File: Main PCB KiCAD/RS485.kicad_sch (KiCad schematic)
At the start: 5 parts, among them J8 RS485, U2 MAX3072E

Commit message: changes adn updates
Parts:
- J8: footprint Connector_Molex:Molex_Nano-Fit_105309-xx08_1x08_P2.50mm_Vertical -> Connector_JST:JST_PH_S8B-PH-K_1x08_P2.00mm_Horizontal
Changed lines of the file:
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@@
 		(dnp no)
 		(fields_autoplaced yes)
-		(property "Reference" "#PWR031"
+		(property "Reference" "#PWR03"
 			(at 217.17 123.19 0)
 			(effects
@@
 		(instances
 			(project "Buoy PCB"
-				(path "/a041e2a6-7d41-458c-91f3-753821d3dfe9/e4da0947-b13f-47c4-af36-48578442859c"
-					(reference "#PWR031")
+				(path "/a041e2a6-7d41-458c-91f3-753821d3dfe9/402c8c5f-ad4a-46d2-a42e-eba9c7fe5855/d9a8ca03-ff66-4db5-998a-66a2672c57da"
+					(reference "#PWR03")
 					(unit 1)
 				)
@@
 		)
 		(instances
-			(project ""
-				(path "/a041e2a6-7d41-458c-91f3-753821d3dfe9/e4da0947-b13f-47c4-af36-48578442859c"
+			(project "Buoy PCB"
+				(path "/a041e2a6-7d41-458c-91f3-753821d3dfe9/402c8c5f-ad4a-46d2-a42e-eba9c7fe5855/d9a8ca03-ff66-4db5-998a-66a2672c57da"
 					(reference "U2")
 					(unit 1)
@@
 		(instances
 			(project "Buoy PCB"
-				(path "/a041e2a6-7d41-458c-91f3-753821d3dfe9/e4da0947-b13f-47c4-af36-48578442859c"
+				(path "/a041e2a6-7d41-458c-91f3-753821d3dfe9/402c8c5f-ad4a-46d2-a42e-eba9c7fe5855/d9a8ca03-ff66-4db5-998a-66a2672c57da"
 					(reference "R7")
 					(unit 1)
@@
 		(instances
 			(project "Buoy PCB"
-				(path "/a041e2a6-7d41-458c-91f3-753821d3dfe9/e4da0947-b13f-47c4-af36-48578442859c"
+				(path "/a041e2a6-7d41-458c-91f3-753821d3dfe9/402c8c5f-ad4a-46d2-a42e-eba9c7fe5855/d9a8ca03-ff66-4db5-998a-66a2672c57da"
 					(reference "JP2")
 					(unit 1)
@@
 		(dnp no)
 		(fields_autoplaced yes)
-		(property "Reference" "#PWR034"
+		(property "Reference" "#PWR032"
 			(at 275.59 151.13 0)
 			(effects
@@
 		(instances
 			(project "Buoy PCB"
-				(path "/a041e2a6-7d41-458c-91f3-753821d3dfe9/e4da0947-b13f-47c4-af36-48578442859c"
-					(reference "#PWR034")
+				(path "/a041e2a6-7d41-458c-91f3-753821d3dfe9/402c8c5f-ad4a-46d2-a42e-eba9c7fe5855/d9a8ca03-ff66-4db5-998a-66a2672c57da"
+					(reference "#PWR032")
 					(unit 1)
 				)
@@
 			)
 		)
-		(property "Footprint" "Connector_Molex:Molex_Nano-Fit_105309-xx08_1x08_P2.50mm_Vertical"
+		(property "Footprint" "Connector_JST:JST_PH_S8B-PH-K_1x08_P2.00mm_Horizontal"
 			(at 283.21 132.08 0)
 			(effects
@@
 		(instances
 			(project "Buoy PCB"
-				(path "/a041e2a6-7d41-458c-91f3-753821d3dfe9/e4da0947-b13f-47c4-af36-48578442859c"
+				(path "/a041e2a6-7d41-458c-91f3-753821d3dfe9/402c8c5f-ad4a-46d2-a42e-eba9c7fe5855/d9a8ca03-ff66-4db5-998a-66a2672c57da"
 					(reference "J8")
 					(unit 1)
@@
 		(instances
 			(project "Buoy PCB"
-				(path "/a041e2a6-7d41-458c-91f3-753821d3dfe9/e4da0947-b13f-47c4-af36-48578442859c"
+				(path "/a041e2a6-7d41-458c-91f3-753821d3dfe9/402c8c5f-ad4a-46d2-a42e-eba9c7fe5855/d9a8ca03-ff66-4db5-998a-66a2672c57da"
 					(reference "JP1")
 					(unit 1)
@@
 		(dnp no)
 		(fields_autoplaced yes)
-		(property "Reference" "#PWR033"
+		(property "Reference" "#PWR031"
 			(at 273.05 118.11 0)
 			(effects
@@
 		(instances
 			(project "Buoy PCB"
-				(path "/a041e2a6-7d41-458c-91f3-753821d3dfe9/e4da0947-b13f-47c4-af36-48578442859c"
-					(reference "#PWR033")
+				(path "/a041e2a6-7d41-458c-91f3-753821d3dfe9/402c8c5f-ad4a-46d2-a42e-eba9c7fe5855/d9a8ca03-ff66-4db5-998a-66a2672c57da"
+					(reference "#PWR031")
 					(unit 1)
 				)
@@
 		(dnp no)
 		(fields_autoplaced yes)
-		(property "Reference" "#PWR032"
+		(property "Reference" "#PWR017"
 			(at 217.17 161.29 0)
 			(effects
@@
 		(instances
 			(project "Buoy PCB"
-				(path "/a041e2a6-7d41-458c-91f3-753821d3dfe9/e4da0947-b13f-47c4-af36-48578442859c"
-					(reference "#PWR032")
-					(unit 1)
-				)
+				(path "/a041e2a6-7d41-458c-91f3-753821d3dfe9/402c8c5f-ad4a-46d2-a42e-eba9c7fe5855/d9a8ca03-ff66-4db5-998a-66a2672c57da"
+					(reference "#PWR017")
+					(unit 1)
+				)

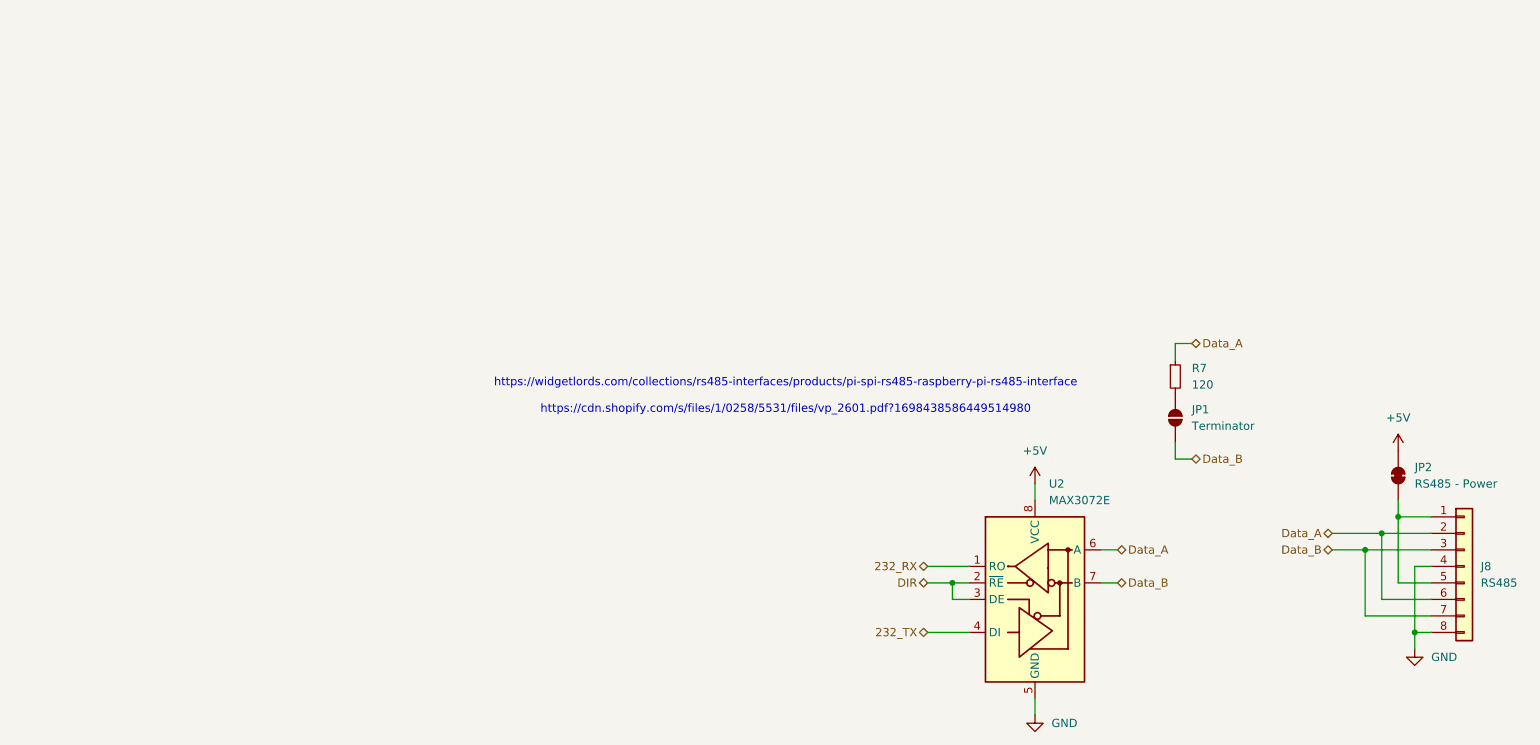
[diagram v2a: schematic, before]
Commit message: .
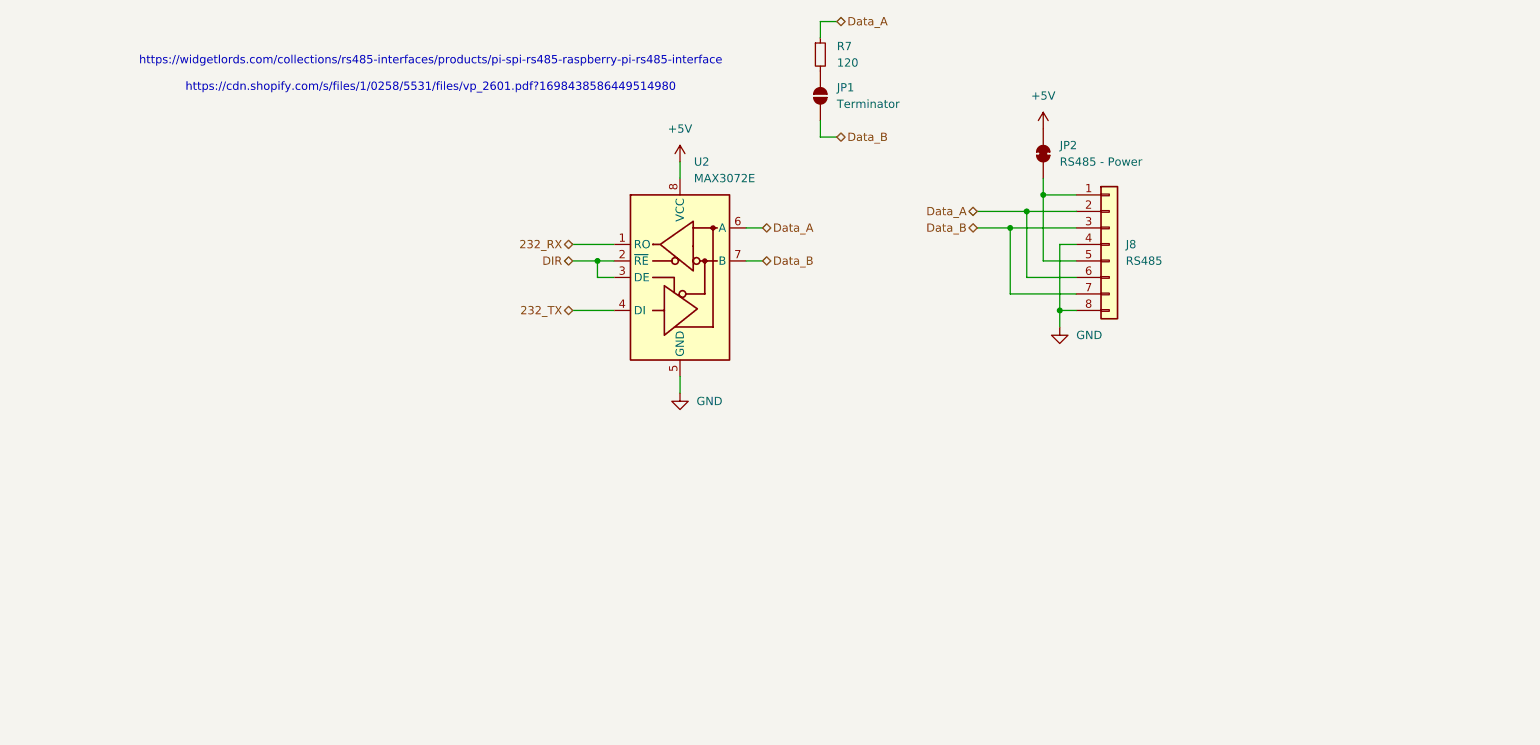
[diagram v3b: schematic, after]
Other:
- moved on the sheet: J8, JP1, JP2, R7, U2

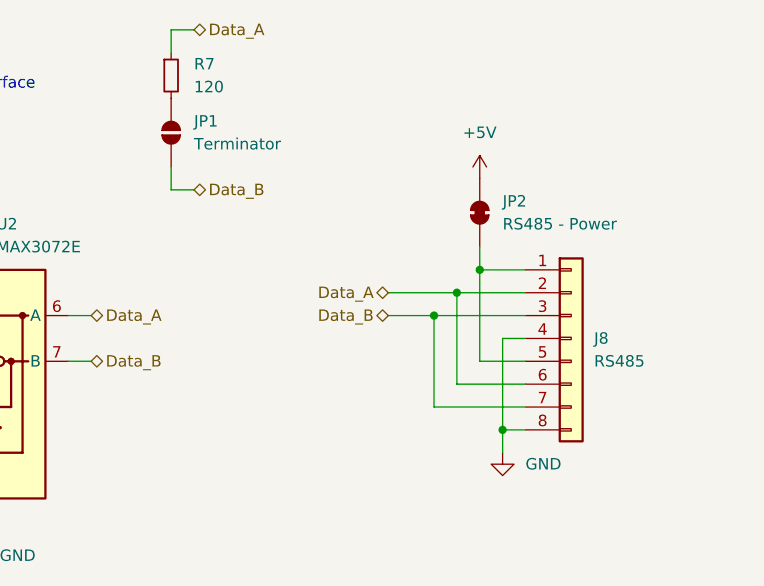
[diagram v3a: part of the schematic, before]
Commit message: .
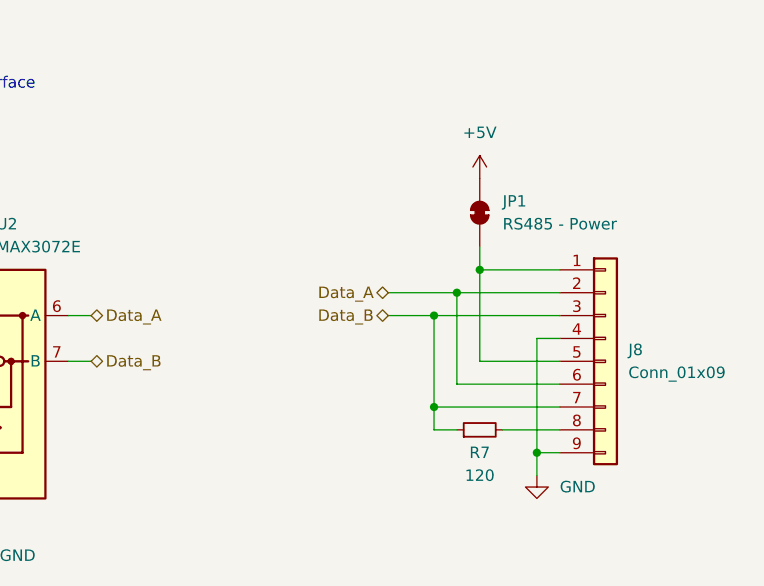
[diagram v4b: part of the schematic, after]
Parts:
- removed JP1: Terminator, Jumper:SolderJumper-2_P1.3mm_Open_RoundedPad1.0x1.5mm, symbol Jumper:SolderJumper_2_Open
- J8: value RS485 -> Conn_01x09; footprint Connector_JST:JST_PH_S8B-PH-K_1x08_P2.00mm_Horizontal -> Connector_JST:JST_EH_S9B-EH_1x09_P2.50mm_Horizontal; symbol Connector_Generic:Conn_01x08 -> Connector_Generic:Conn_01x09
- renumbered JP2 to JP1
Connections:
- net Data_A: no longer R7.1
- net Data_B: now also R7.1
- net GND: now also J8.9 (Pin_9); no longer J8.8 (Pin_8)
- net at R7.2: now also J8.8 (Pin_8)
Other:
- moved on the sheet: R7
